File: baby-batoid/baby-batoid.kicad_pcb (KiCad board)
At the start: 2 copper layers, 20.3 x 50.8 mm, 23 parts, among them J1 USB_C_Receptacle_USB2.0, J2 Conn_01x20, J3 Conn_01x20, U1 STM32F072CBT6, U2 PRTR5V0U2X, U3 XC6206PxxxMR-Regulator_Linear

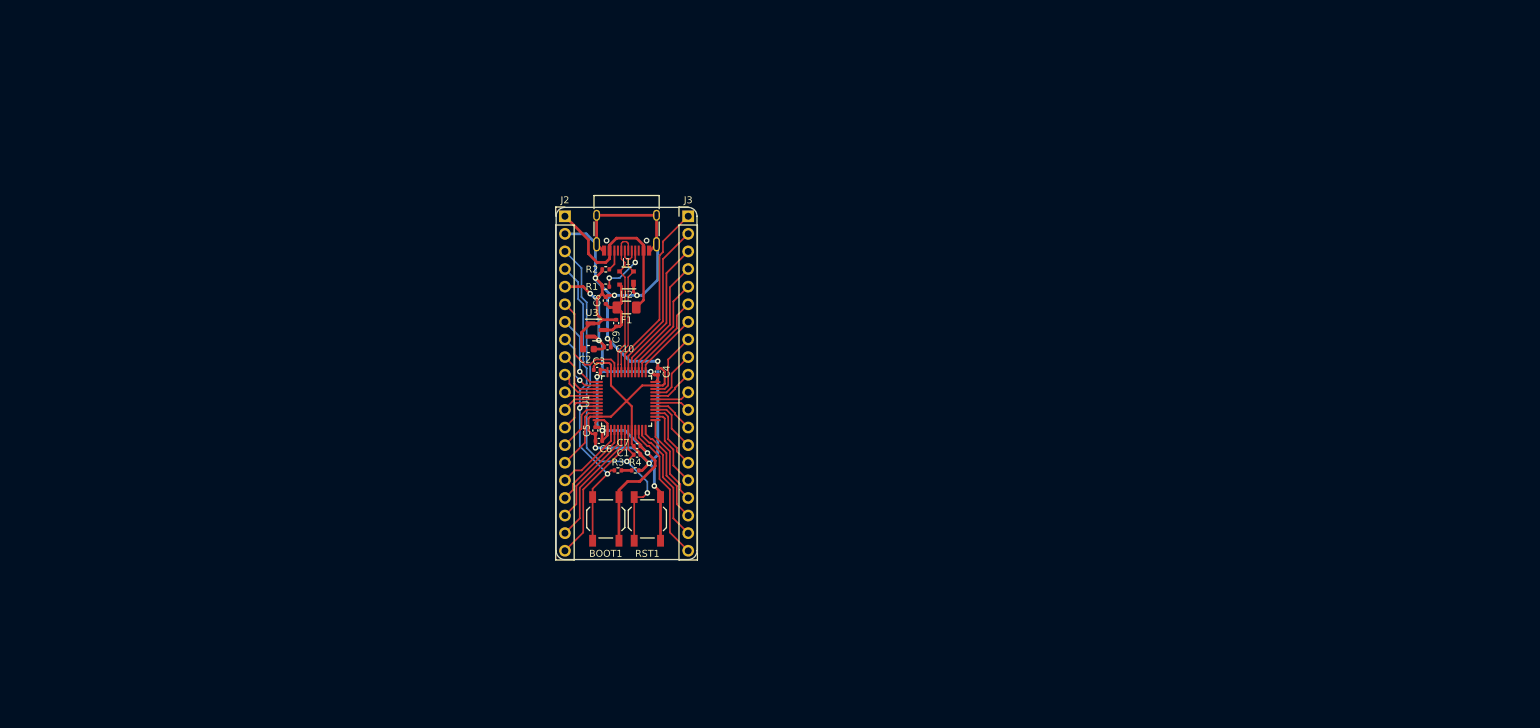
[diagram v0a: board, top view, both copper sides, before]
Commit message: built baby batoid :D
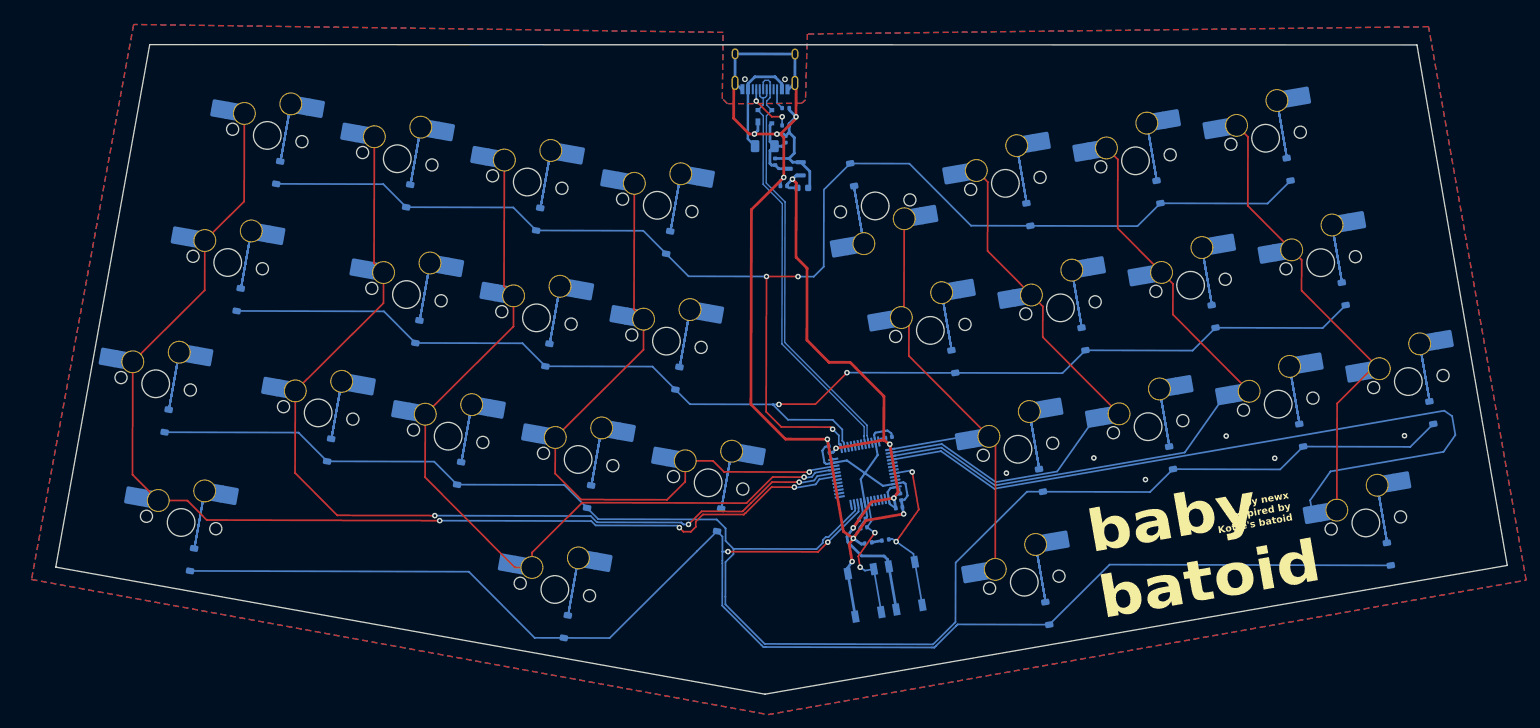
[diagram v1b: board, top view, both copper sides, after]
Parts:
- removed J2, J3: Conn_01x20, Connector_PinHeader_2.54mm:PinHeader_1x20_P2.54mm_Vertical
- added D1: D_Small, Diode_SMD:D_SOD-123, B.Cu at (85.6, 58.9)
- added D10: D_Small, Diode_SMD:D_SOD-123, B.Cu at (93.0, 99.0)
- added D11: D_Small, Diode_SMD:D_SOD-123, B.Cu at (111.7, 102.3)
- added D12: D_Small, Diode_SMD:D_SOD-123, B.Cu at (130.5, 105.7)
- added D13: D_Small, Diode_SMD:D_SOD-123, B.Cu at (149.2, 109.0)
- added D14: D_Small, Diode_SMD:D_SOD-123, B.Cu at (73.2, 114.8)
- added D15: D_Small, Diode_SMD:D_SOD-123, B.Cu at (127.1, 124.4)
- added D16: D_Small, Diode_SMD:D_SOD-123, B.Cu at (168.4, 59.3)
- added D17: D_Small, Diode_SMD:D_SOD-123, B.Cu at (193.9, 65.0)
- added D18: D_Small, Diode_SMD:D_SOD-123, B.Cu at (212.6, 61.7)
- added D19: D_Small, Diode_SMD:D_SOD-123, B.Cu at (231.4, 58.5)
- added D2: D_Small, Diode_SMD:D_SOD-123, B.Cu at (104.4, 62.3)
- added D20: D_Small, Diode_SMD:D_SOD-123, B.Cu at (183.0, 86.2)
- added D21: D_Small, Diode_SMD:D_SOD-123, B.Cu at (201.8, 83.0)
- added D22: D_Small, Diode_SMD:D_SOD-123, B.Cu at (220.6, 79.7)
- added D23: D_Small, Diode_SMD:D_SOD-123, B.Cu at (239.3, 76.4)
- added D24: D_Small, Diode_SMD:D_SOD-123, B.Cu at (195.7, 103.3)
- added D25: D_Small, Diode_SMD:D_SOD-123, B.Cu at (214.4, 100.1)
- added D26: D_Small, Diode_SMD:D_SOD-123, B.Cu at (233.2, 96.8)
- added D27: D_Small, Diode_SMD:D_SOD-123, B.Cu at (252.0, 93.6)
- added D28: D_Small, Diode_SMD:D_SOD-123, B.Cu at (196.6, 122.5)
- added D29: D_Small, Diode_SMD:D_SOD-123, B.Cu at (245.9, 114.0)
- added D3: D_Small, Diode_SMD:D_SOD-123, B.Cu at (123.1, 65.7)
- added D4: D_Small, Diode_SMD:D_SOD-123, B.Cu at (141.9, 69.0)
- added D5: D_Small, Diode_SMD:D_SOD-123, B.Cu at (79.9, 77.3)
- added D6: D_Small, Diode_SMD:D_SOD-123, B.Cu at (105.7, 81.9)
- added D7: D_Small, Diode_SMD:D_SOD-123, B.Cu at (124.5, 85.3)
- added D8: D_Small, Diode_SMD:D_SOD-123, B.Cu at (143.2, 88.6)
- added D9: D_Small, Diode_SMD:D_SOD-123, B.Cu at (69.5, 94.8)
- added MX1: MX_SW_HS, marbastlib-mx:SW_MX_HS_CPG151101S11_1u, B.Cu at (84.1, 53.6)
- added MX10: MX_SW_HS, marbastlib-mx:SW_MX_HS_CPG151101S11_1u, B.Cu at (91.4, 93.6)
- added MX11: MX_SW_HS, marbastlib-mx:SW_MX_HS_CPG151101S11_1u, B.Cu at (110.2, 97.0)
- added MX12: MX_SW_HS, marbastlib-mx:SW_MX_HS_CPG151101S11_1u, B.Cu at (128.9, 100.3)
- added MX13: MX_SW_HS, marbastlib-mx:SW_MX_HS_CPG151101S11_1u, B.Cu at (147.7, 103.7)
- added MX14: MX_SW_HS, marbastlib-mx:SW_MX_HS_CPG151101S11_1u, B.Cu at (71.6, 109.4)
- added MX15: MX_SW_HS, marbastlib-mx:SW_MX_HS_CPG151101S11_1u, B.Cu at (125.5, 119.1)
- added MX16: MX_SW_HS, marbastlib-mx:SW_MX_HS_CPG151101S11_1u, B.Cu at (171.8, 63.8)
- added MX17: MX_SW_HS, marbastlib-mx:SW_MX_HS_CPG151101S11_1u, B.Cu at (190.5, 60.5)
- added MX18: MX_SW_HS, marbastlib-mx:SW_MX_HS_CPG151101S11_1u, B.Cu at (209.3, 57.2)
- added MX19: MX_SW_HS, marbastlib-mx:SW_MX_HS_CPG151101S11_1u, B.Cu at (228.1, 54.0)
- added MX2: MX_SW_HS, marbastlib-mx:SW_MX_HS_CPG151101S11_1u, B.Cu at (102.8, 56.9)
- added MX20: MX_SW_HS, marbastlib-mx:SW_MX_HS_CPG151101S11_1u, B.Cu at (179.7, 81.7)
- added MX21: MX_SW_HS, marbastlib-mx:SW_MX_HS_CPG151101S11_1u, B.Cu at (198.5, 78.5)
- added MX22: MX_SW_HS, marbastlib-mx:SW_MX_HS_CPG151101S11_1u, B.Cu at (217.3, 75.2)
- added MX23: MX_SW_HS, marbastlib-mx:SW_MX_HS_CPG151101S11_1u, B.Cu at (236.0, 71.9)
- added MX24: MX_SW_HS, marbastlib-mx:SW_MX_HS_CPG151101S11_1u, B.Cu at (192.4, 98.8)
- added MX25: MX_SW_HS, marbastlib-mx:SW_MX_HS_CPG151101S11_1u, B.Cu at (211.1, 95.6)
- added MX26: MX_SW_HS, marbastlib-mx:SW_MX_HS_CPG151101S11_1u, B.Cu at (229.9, 92.3)
- added MX27: MX_SW_HS, marbastlib-mx:SW_MX_HS_CPG151101S11_1u, B.Cu at (248.7, 89.1)
- added MX28: MX_SW_HS, marbastlib-mx:SW_MX_HS_CPG151101S11_1u, B.Cu at (193.3, 118.0)
- added MX29: MX_SW_HS, marbastlib-mx:SW_MX_HS_CPG151101S11_1u, B.Cu at (242.5, 109.5)
- added MX3: MX_SW_HS, marbastlib-mx:SW_MX_HS_CPG151101S11_1u, B.Cu at (121.6, 60.3)
- added MX4: MX_SW_HS, marbastlib-mx:SW_MX_HS_CPG151101S11_1u, B.Cu at (140.3, 63.7)
- added MX5: MX_SW_HS, marbastlib-mx:SW_MX_HS_CPG151101S11_1u, B.Cu at (78.4, 71.9)
- added MX6: MX_SW_HS, marbastlib-mx:SW_MX_HS_CPG151101S11_1u, B.Cu at (104.1, 76.5)
- added MX7: MX_SW_HS, marbastlib-mx:SW_MX_HS_CPG151101S11_1u, B.Cu at (122.9, 79.9)
- added MX8: MX_SW_HS, marbastlib-mx:SW_MX_HS_CPG151101S11_1u, B.Cu at (141.6, 83.3)
- added MX9: MX_SW_HS, marbastlib-mx:SW_MX_HS_CPG151101S11_1u, B.Cu at (68.0, 89.4)
- BOOT1, C1, C10, C2, C3, C4, C5, C6, C7, C8, C9, F1, J1, R1, R2, R3, R4, RST1, U1, U2, U3: moved to B.Cu
- moved C5 45.1 mm to (175.4, 105.7), turned to -80.16 degrees
- moved C6 44.4 mm to (175.2, 107.3), turned to 9.84 degrees
- moved BOOT1 44.3 mm to (176.1, 118.5), turned to -80.16 degrees
- moved C3 43.2 mm to (173.7, 97.1), turned to 9.84 degrees
- moved R3 39.9 mm to (173.2, 111.9), turned to -170.16 degrees
- moved C2 38.7 mm to (161.3, 61.1), turned to -0.16 degrees
- moved U3 36.7 mm to (160.1, 58.4), turned to 179.84 degrees
- moved U1 35.9 mm to (170.3, 102.3), turned to 99.84 degrees
- moved R4 35.2 mm to (170.8, 112.4), turned to -170.16 degrees
- moved R2 34.9 mm to (158.8, 49.6), turned to -0.16 degrees
- moved R1 34.8 mm to (158.8, 52.1), turned to 179.84 degrees
- moved C8 34.8 mm to (158.8, 54.1), turned to 89.84 degrees
- moved C10 34.5 mm to (158.6, 60.9), turned to 179.84 degrees
- moved C1 34.4 mm to (170.1, 110.2), turned to -170.16 degrees
- moved C7 34.2 mm to (169.9, 109.0), turned to 9.84 degrees
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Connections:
- U1 pad 10: /A0 -> ROW3
- U1 pad 11: /A1 -> ROW2
- U1 pad 19: /B1 -> COL0
- U1 pad 20: /B2 -> COL1
- U1 pad 21: /B10 -> COL2
- U1 pad 22: /B11 -> COL3
- U1 pad 25: /B12 -> ROW0
- U1 pad 26: /B13 -> ROW1
- U1 pad 37: /A14 -> COL4
- U1 pad 38: /A15 -> COL5
- U1 pad 39: /B3 -> COL6
- U1 pad 40: /B4 -> COL7
- U2 pad 2: D_N -> D-
- U2 pad 3: D_P -> D+
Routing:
- net ROW2: track 0.00 -> 241.5 mm
- net ROW3: track 0.00 -> 223.7 mm, vias 0 -> 2
- net ROW0: track 0.00 -> 204.7 mm, vias 0 -> 3
- net ROW1: track 0.00 -> 185.0 mm, vias 0 -> 2
- net COL7: track 0.00 -> 180.4 mm
- net COL0: track 0.00 -> 167.2 mm, vias 0 -> 3
- net COL1: track 0.00 -> 138.3 mm, vias 0 -> 3
- net COL2: track 0.00 -> 123.2 mm, vias 0 -> 1
- net COL6: track 0.00 -> 98.2 mm
- net COL3: track 0.00 -> 94.5 mm, vias 0 -> 1
- net COL5: track 0.00 -> 79.0 mm
- net COL4: track 0.00 -> 67.4 mm
- net D+: track 0.00 -> 61.2 mm
- net Net-(D28-K): track 0.00 -> 59.9 mm
- net Net-(D7-K): track 0.00 -> 59.9 mm
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- added copper zone on B.Cu, net GND
- added copper zone on F.Cu, net GND
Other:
- board size 20.3 x 50.8 mm -> 209.4 x 93.7 mm
- board text added: "baby batoid"
- board text added: "by newx inspired by Kotte's batoid"

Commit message: production file work
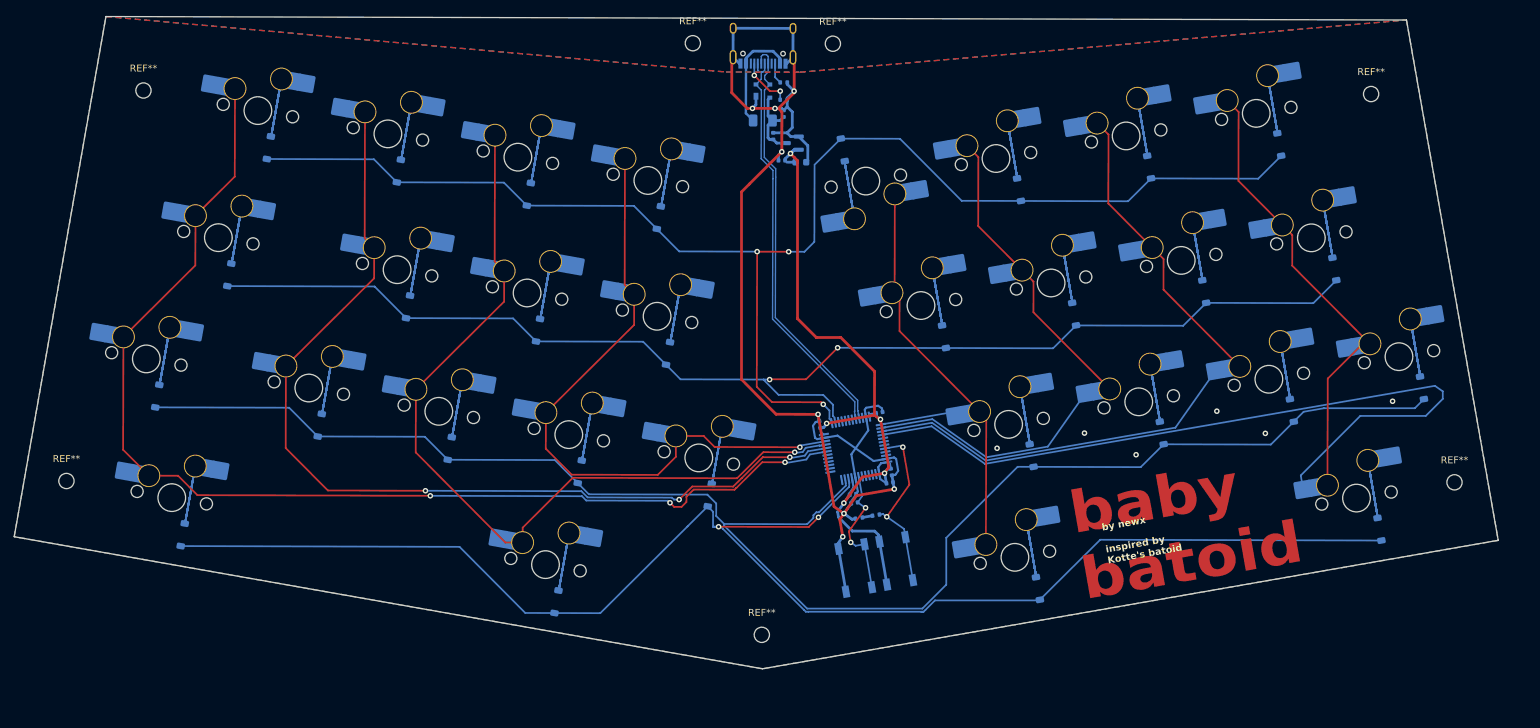
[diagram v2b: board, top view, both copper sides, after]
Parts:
- added REF**: MountingHole_2.2mm_M2, MountingHole:MountingHole_2.2mm_M2, F.Cu at (66.2, 47.1)
- added REF**: MountingHole_2.2mm_M2, MountingHole:MountingHole_2.2mm_M2, F.Cu at (55.1, 103.4)
- added REF**: MountingHole_2.2mm_M2, MountingHole:MountingHole_2.2mm_M2, F.Cu at (155.4, 125.6)
- added REF**: MountingHole_2.2mm_M2, MountingHole:MountingHole_2.2mm_M2, F.Cu at (145.5, 40.3)
- added REF**: MountingHole_2.2mm_M2, MountingHole:MountingHole_2.2mm_M2, F.Cu at (243.3, 47.6)
- added REF**: MountingHole_2.2mm_M2, MountingHole:MountingHole_2.2mm_M2, F.Cu at (255.3, 103.6)
- added REF**: MountingHole_2.2mm_M2, MountingHole:MountingHole_2.2mm_M2, F.Cu at (165.7, 40.4)
- MX5: footprint marbastlib-mx:SW_MX_HS_CPG151101S11_1u -> marbastlib-mx:SW_MX_HS_CPG151101S11_1.75u
- MX9: footprint marbastlib-mx:SW_MX_HS_CPG151101S11_1u -> marbastlib-mx:SW_MX_HS_CPG151101S11_1.5u
- moved D18 3.83 mm to (211.3, 58.2)
- moved C6 3.83 mm to (173.9, 103.7)
- moved MX23 3.83 mm to (234.7, 68.4)
- moved MX28 3.83 mm to (191.9, 114.4)
- moved D21 3.83 mm to (200.5, 79.4)
- moved D27 3.83 mm to (250.6, 90.0)
- moved MX11 3.83 mm to (108.8, 93.4)
- moved MX19 3.83 mm to (226.7, 50.4)
- moved D29 3.83 mm to (244.5, 110.4)
- moved MX15 3.83 mm to (124.2, 115.5)
- moved D3 3.83 mm to (121.8, 62.1)
- moved MX13 3.83 mm to (146.3, 100.1)
- moved MX14 3.83 mm to (70.3, 105.8)
- moved BOOT1 3.83 mm to (174.8, 115.0)
- moved MX29 3.83 mm to (241.2, 105.9)
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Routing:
- net ROW2: track 241.5 -> 232.8 mm
- net ROW3: track 223.7 -> 217.9 mm
- net COL7: track 180.4 -> 179.2 mm
- net GND: track 196.5 -> 197.1 mm
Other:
- board size 209.4 x 93.7 mm -> 214.1 x 94.1 mm
